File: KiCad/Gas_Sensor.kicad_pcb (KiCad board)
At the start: 2 copper layers, 59.1 x 54.6 mm, 18 parts, among them J1 Conn_01x07, Q1 IRF520, SW1 SW_SPDT, U1 Capteur_Gaz, U3 MCP41100

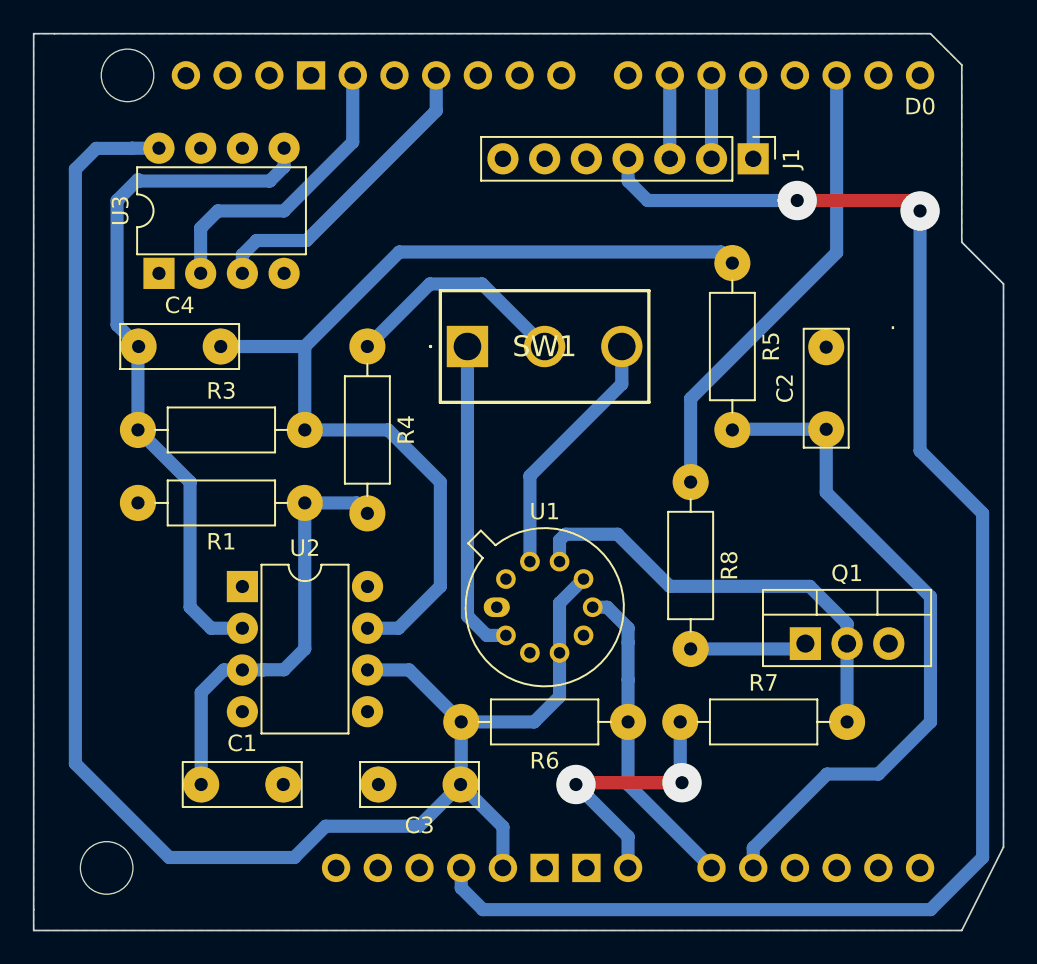
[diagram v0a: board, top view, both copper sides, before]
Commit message: README update
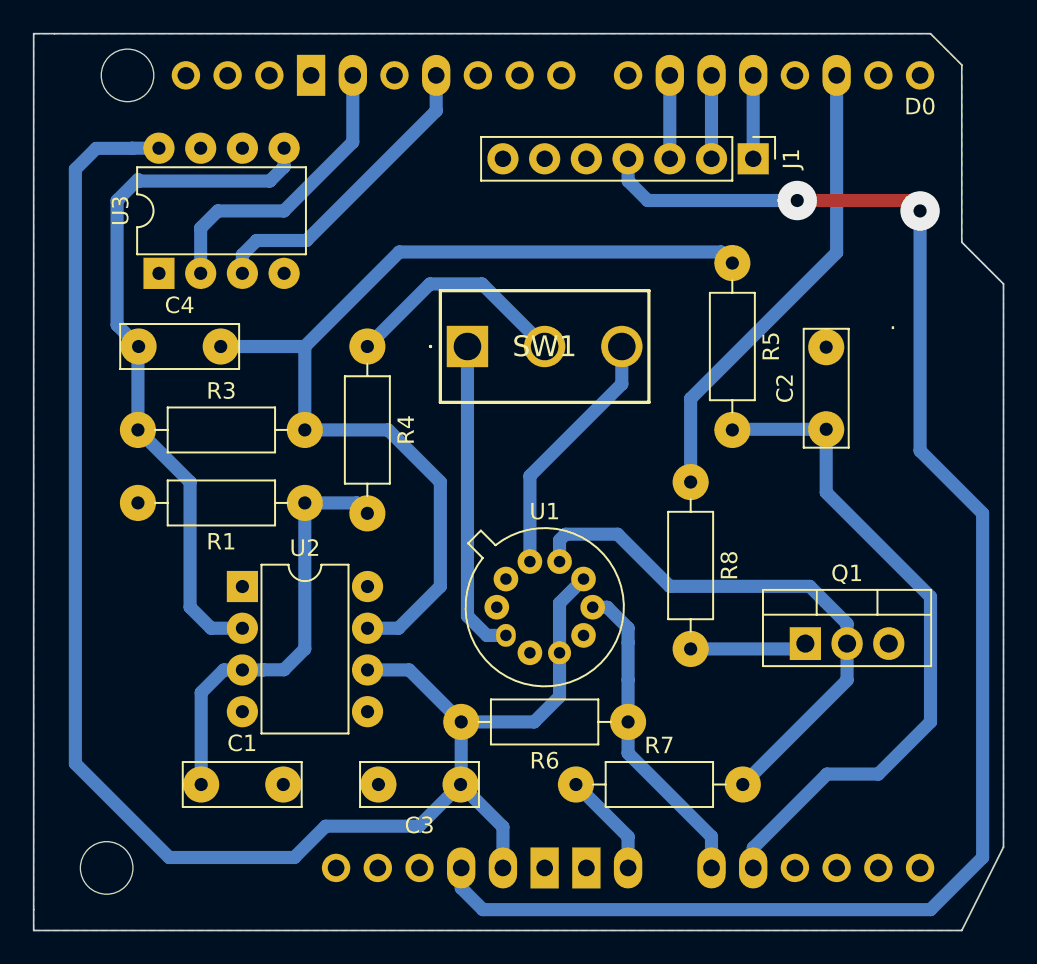
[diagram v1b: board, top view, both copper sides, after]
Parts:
- moved R7 7.41 mm to (71.1, 62.2)
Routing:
- net +12V: track 16.6 -> 6.40 mm, vias 2 -> 0
- net SW_12V: track 27.2 -> 33.6 mm
